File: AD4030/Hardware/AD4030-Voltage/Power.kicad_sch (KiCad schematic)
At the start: 64 parts, among them J501 1715721, Q501 SI5618A, Q502 MMBT3904, U501 TSR_1-2450, U502 ADP5070AREZ, U503 TSR_1-2433, U504 LT3032-5, U505 TSR_1-2433, U506 TEC3-2419WI, U507 LT1763CS8-ADJ, U508 LT1763CS8-1.8, U509 LT1763CS8-1.8

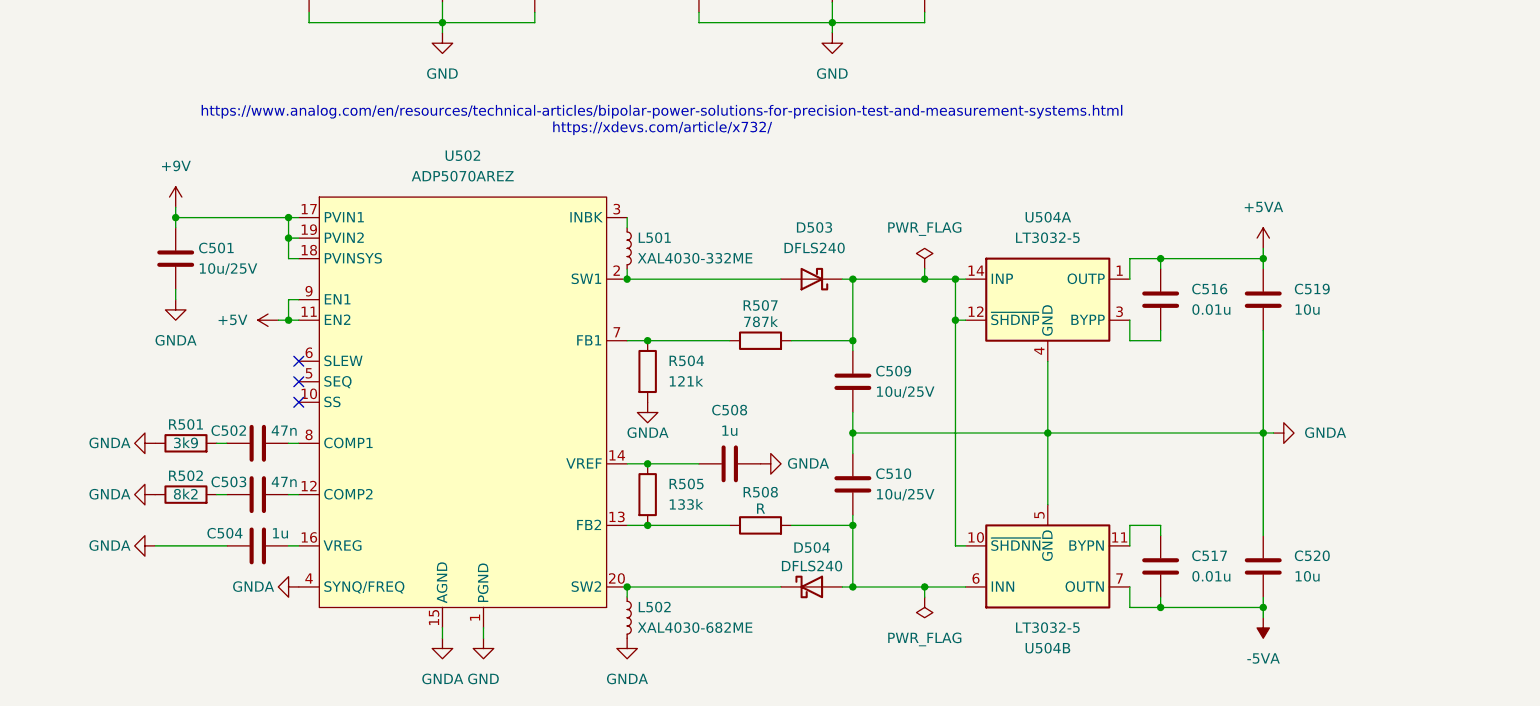
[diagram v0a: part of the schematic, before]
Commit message: Hardware
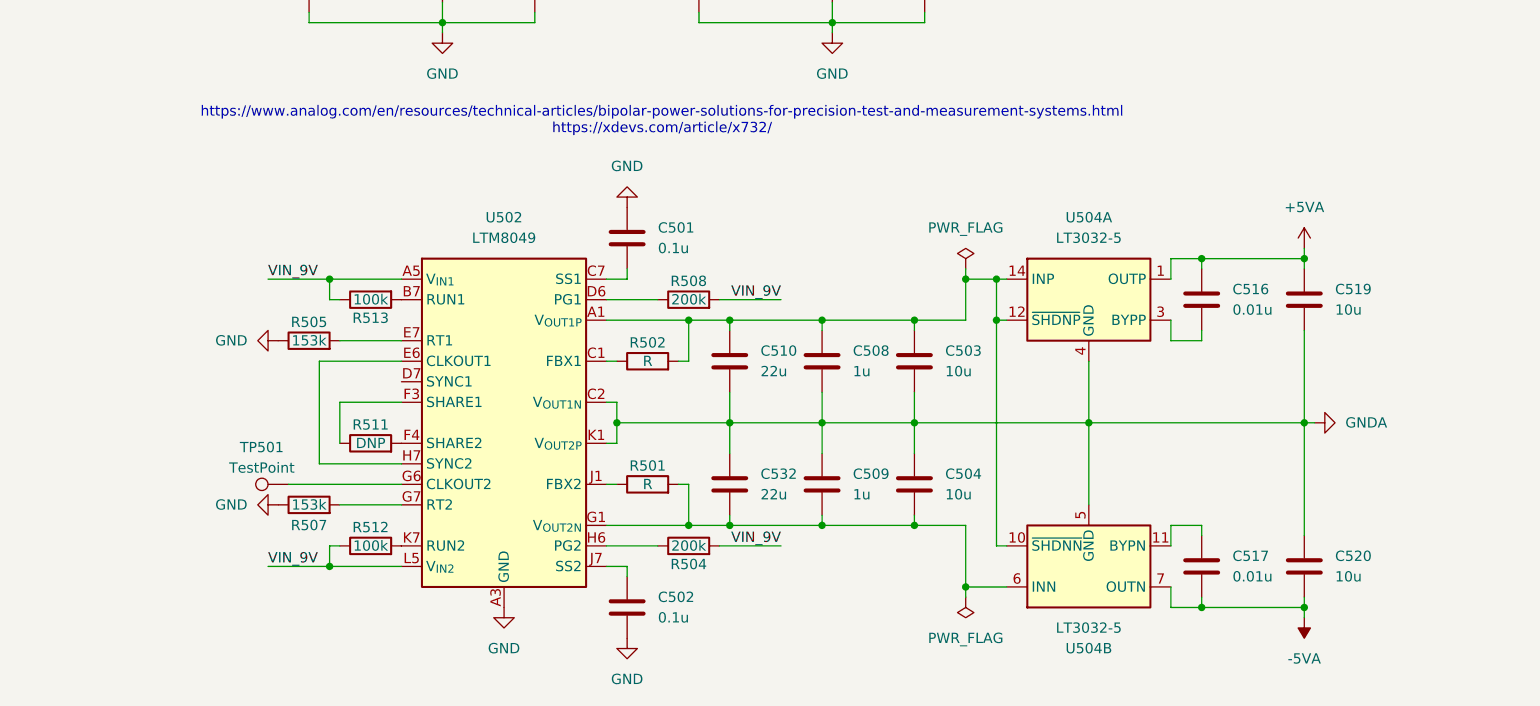
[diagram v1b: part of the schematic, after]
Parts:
- removed D503, D504: DFLS240, AD4030:POWERDI123_DIO, symbol Device:D_Schottky
- removed L501: XAL4030-332ME, AD4030:XAL4030, symbol Device:L_Small
- removed L502: XAL4030-682ME, AD4030:XAL4030, symbol Device:L_Small
- removed U502: ADP5070AREZ, Package_SO:ETSSOP-20-1EP_4.4x6.5mm_P0.65mm_EP3x4.2mm, symbol AD4030:ADP5070AREZ
- added C532: 22u, symbol Device:C
- added R511: DNP, symbol Device:R
- added R512, R513: 100k, symbol Device:R
- added TP501: TestPoint, symbol Connector:TestPoint
- added U502: LTM8049, Package_BGA:Analog_BGA-77_9.0x15.0mm_Layout7x11_P1.27mm_Ball0.63mm, symbol Regulator_Switching:LTM8049
- C501: value 10u/25V -> 0.1u; footprint Capacitor_SMD:C_1206_3216Metric_Pad1.33x1.80mm_HandSolder -> (none)
- C502: value 47n -> 0.1u; footprint Capacitor_SMD:C_0603_1608Metric_Pad1.08x0.95mm_HandSolder -> (none)
- C503: value 47n -> 10u; footprint Capacitor_SMD:C_0603_1608Metric_Pad1.08x0.95mm_HandSolder -> Capacitor_SMD:C_1206_3216Metric_Pad1.33x1.80mm_HandSolder
- C504: value 1u -> 10u; footprint Capacitor_SMD:C_0603_1608Metric_Pad1.08x0.95mm_HandSolder -> Capacitor_SMD:C_1206_3216Metric_Pad1.33x1.80mm_HandSolder
- C508: footprint Capacitor_SMD:C_0603_1608Metric_Pad1.08x0.95mm_HandSolder -> (none)
- C509: value 10u/25V -> 1u; footprint Capacitor_SMD:C_1206_3216Metric_Pad1.33x1.80mm_HandSolder -> (none)
- C510: value 10u/25V -> 22u; footprint Capacitor_SMD:C_1206_3216Metric_Pad1.33x1.80mm_HandSolder -> (none)
- R501: value 3k9 -> R; footprint Resistor_SMD:R_0603_1608Metric_Pad0.98x0.95mm_HandSolder -> (none)
- R502: value 8k2 -> R; footprint Resistor_SMD:R_0603_1608Metric_Pad0.98x0.95mm_HandSolder -> (none)
- R504: value 121k -> 200k; footprint Resistor_SMD:R_0603_1608Metric_Pad0.98x0.95mm_HandSolder -> (none)
- R505: value 133k -> 153k; footprint Resistor_SMD:R_0603_1608Metric_Pad0.98x0.95mm_HandSolder -> (none)
- R507: value 787k -> 153k; footprint Resistor_SMD:R_0603_1608Metric_Pad0.98x0.95mm_HandSolder -> (none)
- R508: value R -> 200k; footprint Resistor_SMD:R_0603_1608Metric_Pad0.98x0.95mm_HandSolder -> (none)
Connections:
- net +9V: no longer C501.1
- net GND: now also C501.1, C502.2, C503.2, C509.1, C510.2, R505.1, R507.1, C532.1, U502.A3 (GND), U502.A4 (GND), U502.B3 (GND), U502.B4 (GND), U502.B5 (GND), U502.B6 (GND), U502.C2 (V_{OUT1N}), U502.C3 (GND), U502.C4 (GND), U502.C5 (GND), U502.C6 (GND), U502.D1 (V_{OUT1N}), U502.D2 (V_{OUT1N}), U502.D3 (GND), U502.D4 (GND), U502.D5 (GND), U502.E1 (V_{OUT1N}), U502.E2 (V_{OUT1N}), U502.E3 (GND), U502.E4 (GND), U502.E5 (GND), U502.F1 (GND), U502.F2 (GND), U502.F5 (GND), U502.F6 (GND), U502.F7 (GND), U502.G3 (GND), U502.G4 (GND), U502.G5 (GND), U502.H3 (GND), U502.H4 (GND), U502.H5 (GND), U502.J3 (GND), U502.J4 (GND), U502.J5 (GND), U502.J6 (GND), U502.K1 (V_{OUT2P}), U502.K2 (V_{OUT2P}), U502.K3 (GND), U502.K4 (GND), U502.K5 (GND), U502.K6 (GND), U502.L1 (V_{OUT2P}), U502.L2 (V_{OUT2P}), U502.L3 (GND), U502.L4 (GND); no longer C501.2, C509.2, C510.1, R501.1, R502.1, R504.2
- net at C503.1, R502.2: now also C508.1, C510.1, U504.10 (~{SHDNN}), U504.12 (~{SHDNP}), U504.14 (INP), U502.A1 (V_{OUT1P}), U502.A2 (V_{OUT1P}), U502.B1 (V_{OUT1P}), U502.B2 (V_{OUT1P})
- net at R501.2: now also C504.2, C509.2, U504.6 (INN), U504.9 (INN), C532.2, U502.G1 (V_{OUT2N}), U502.G2 (V_{OUT2N}), U502.H1 (V_{OUT2N}), U502.H2 (V_{OUT2N}), U502.J2 (V_{OUT2N}); no longer C502.1
- net at R505.2: now also U502.E7 (RT1); no longer R508.1
- net at R504.1: now also U502.H6 (PG2); no longer R507.1
- new net: R507.2, U502.G7 (RT2)
- new net: R502.1, U502.C1 (FBX1)
- new net: TP501.1, U502.G6 (CLKOUT2)
- new net: R512.2, U502.K7 (RUN2)
- new net: R511.1, U502.F3 (SHARE1)
- new net: R511.2, U502.F4 (SHARE2)
- new net: R501.1, U502.J1 (FBX2)
- new net: R513.2, U502.B7 (RUN1)
- new net: R508.1, U502.D6 (PG1)
- new net: C502.1, U502.J7 (SS2)
- new net: C501.2, U502.C7 (SS1)
- new net: U502.E6 (CLKOUT1), U502.H7 (SYNC2)
- new net VIN_9V: R504.2, R508.2, R512.1, R513.1, U502.A5 (V_{IN1}), U502.A6 (V_{IN1}), U502.A7 (V_{IN1}), U502.L5 (V_{IN2}), U502.L6 (V_{IN2}), U502.L7 (V_{IN2})
- no-connect marks 4 -> 1
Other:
- moved on the sheet: C516, C517, C519, C520, U504A, U504B

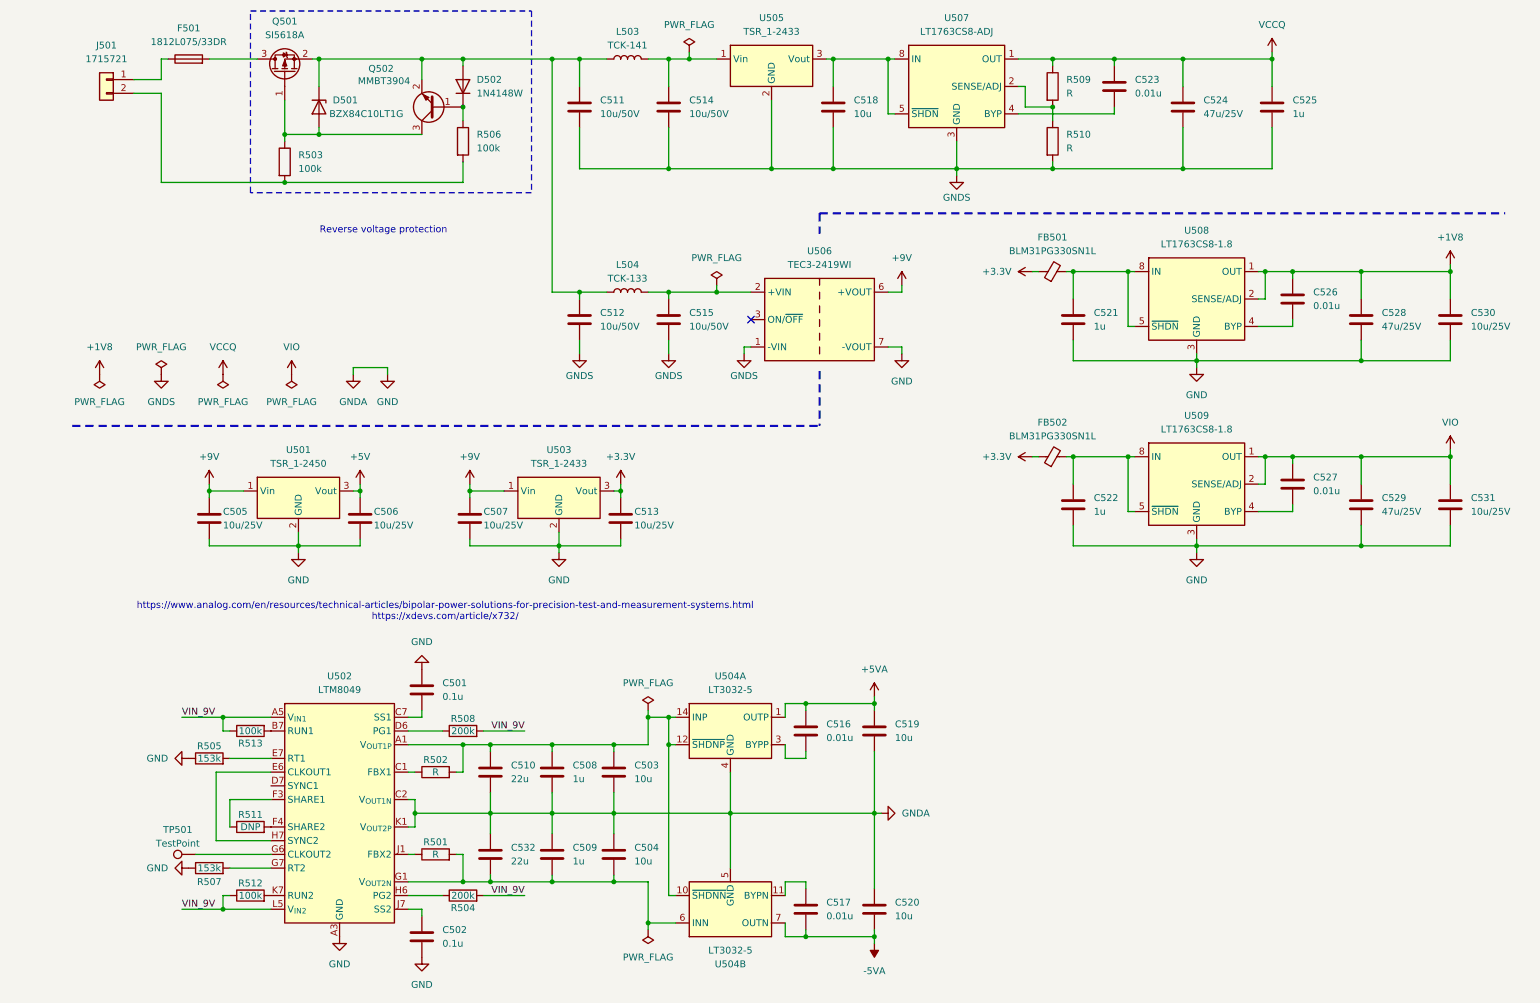
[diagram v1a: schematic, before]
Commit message: Hardware and update to 2024.1
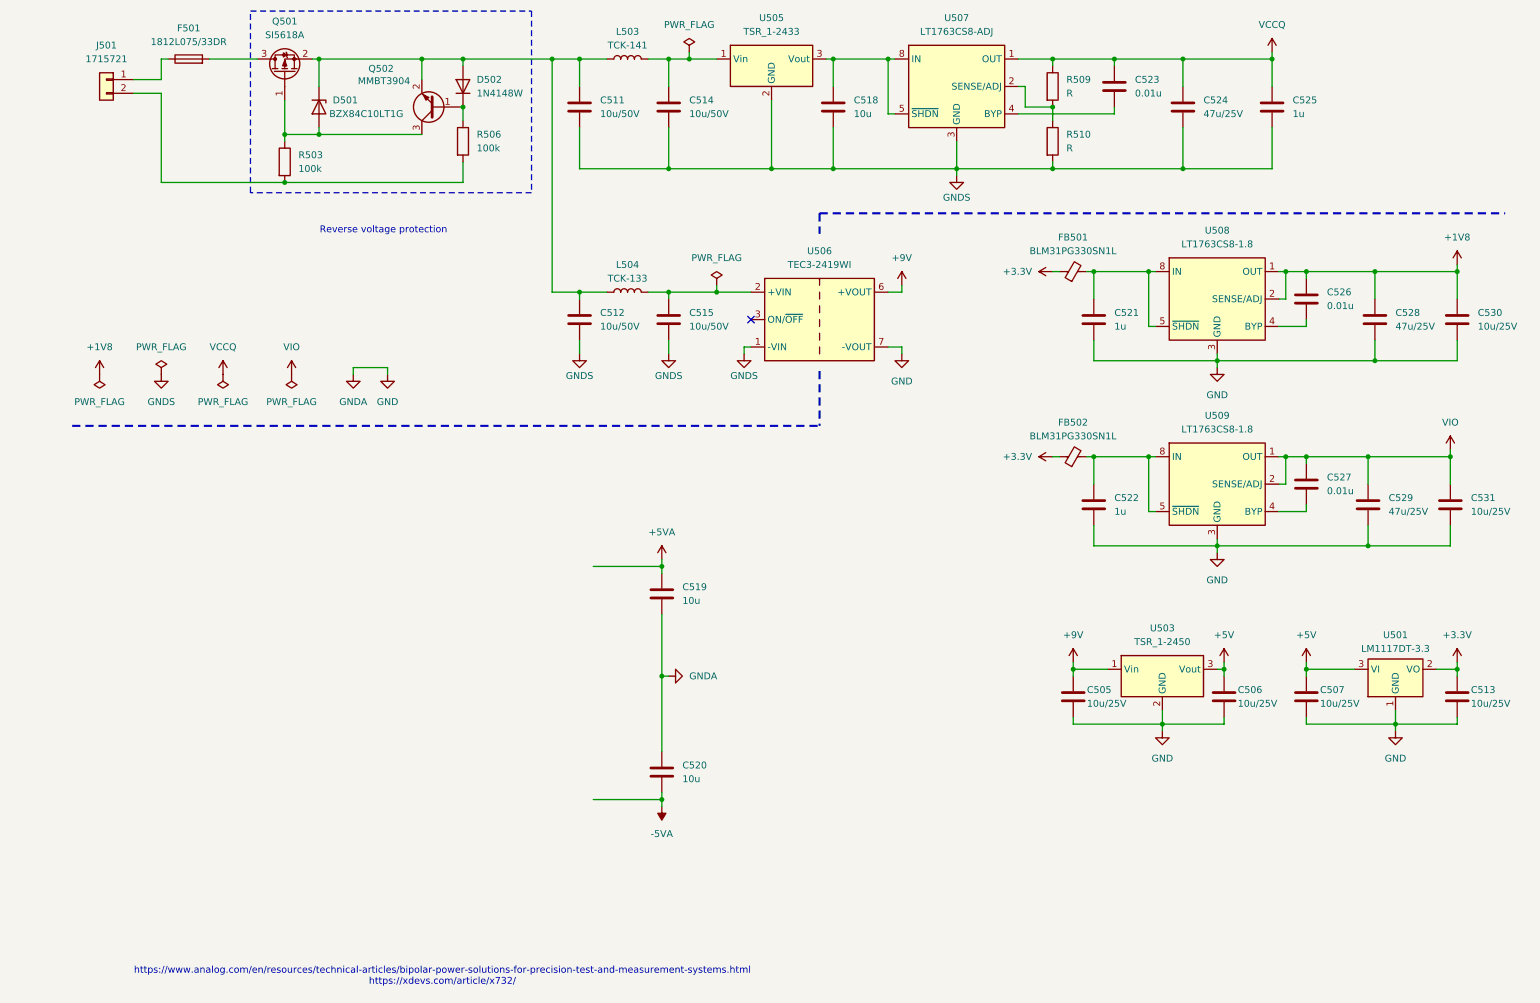
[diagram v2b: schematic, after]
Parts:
- removed C501, C502: 0.1u, symbol Device:C
- removed C503, C504: 10u, Capacitor_SMD:C_1206_3216Metric_Pad1.33x1.80mm_HandSolder, symbol Device:C
- removed C508, C509: 1u, symbol Device:C
- removed C510, C532: 22u, symbol Device:C
- removed C516, C517: 0.01u, Capacitor_SMD:C_0603_1608Metric_Pad1.08x0.95mm_HandSolder, symbol Device:C
- removed R501, R502: R, symbol Device:R
- removed R504, R508: 200k, symbol Device:R
- removed R505, R507: 153k, symbol Device:R
- removed R511: DNP, symbol Device:R
- removed R512, R513: 100k, symbol Device:R
- removed TP501: TestPoint, symbol Connector:TestPoint
- removed U501: TSR_1-2450, Converter_DCDC:Converter_DCDC_TRACO_TSR-1_THT, symbol Regulator_Switching:TSR_1-2450
- removed U502: LTM8049, Package_BGA:Analog_BGA-77_9.0x15.0mm_Layout7x11_P1.27mm_Ball0.63mm, symbol Regulator_Switching:LTM8049
- removed U503: TSR_1-2433, Converter_DCDC:Converter_DCDC_TRACO_TSR-1_THT, symbol Regulator_Switching:TSR_1-2433
- removed U504: LT3032-5, Package_DFN_QFN:Linear_DE14MA, symbol Regulator_Linear:LT3032-5
- added U501: LM1117DT-3.3, Package_TO_SOT_SMD:TO-252-3_TabPin2, symbol Regulator_Linear:LM1117DT-3.3
- added U503: TSR_1-2450, Converter_DCDC:Converter_DCDC_TRACO_TSR-1_THT, symbol Regulator_Switching:TSR_1-2450
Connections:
- net +3.3V: now also U501.2 (VO)
- net +5V: now also C507.1, U501.3 (VI), U503.3 (Vout)
- net +9V: now also U503.1 (Vin); no longer C507.1
- net GND: now also U501.1 (GND), U503.2 (GND)
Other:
- moved on the sheet: C505, C506, C507, C513, C519, C520, C521, C522, C526, C527, C528, C529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
